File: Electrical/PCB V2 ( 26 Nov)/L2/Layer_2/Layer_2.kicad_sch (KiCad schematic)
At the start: 25 parts, among them SW1 SW_Push, U1 LM2596ADJ, U2 LM2596ADJ, U3 XT30UPB-M, U4 XT30UPB-M, U5 ESP32-S3-DEVKITM-1-N8, U6 XT30UPB-M, U7 XT30UPB-M, U8 XT30UPB-M, U9 XT30UPB-M

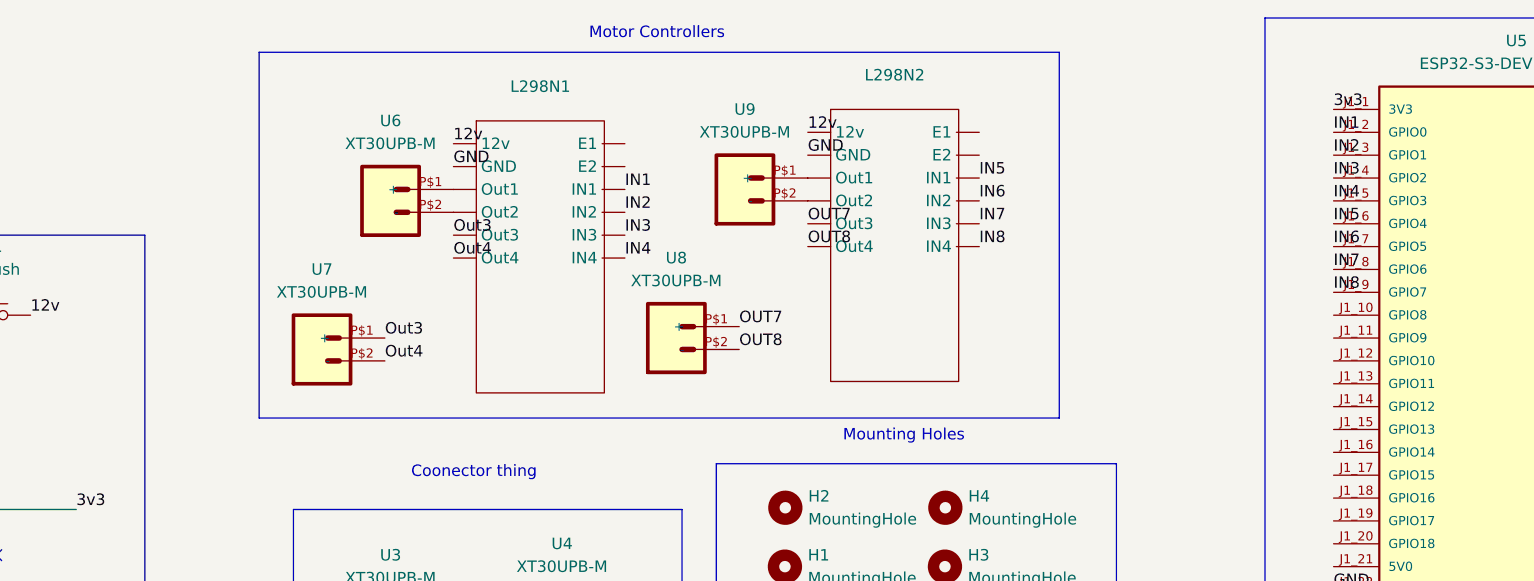
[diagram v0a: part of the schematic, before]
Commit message: concern
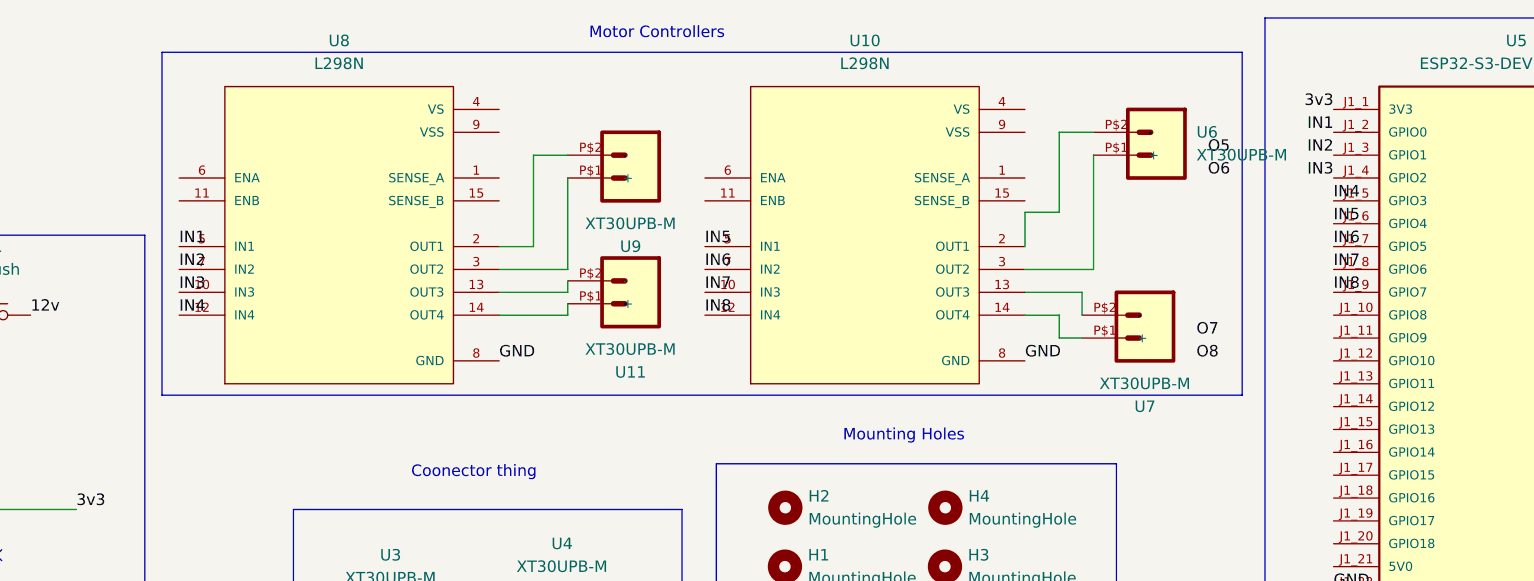
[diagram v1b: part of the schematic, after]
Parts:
- removed L298N1, L298N2: ~, l298n:TO127P2020X500X2100-15, symbol motor driver:L298N
- removed U8: XT30UPB-M, xt30:XT30UPB-M, symbol XT30UPB-M:XT30UPB-M
- added U10, U8: L298N, L298N:TO127P2020X500X2100-15, symbol l298n:L298N
- added U11: XT30UPB-M, xt30:XT30UPB-M, symbol XT30UPB-M:XT30UPB-M
- U3, U4: footprint XT30UPB-M:XT30UPB-M -> xt30:XT30UPB-M
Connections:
- net GND: now also U10.8 (GND), U8.8 (GND)
- net IN1: now also U8.5 (IN1)
- net IN2: now also U8.7 (IN2)
- net IN3: now also U8.10 (IN3)
- net IN4: now also U8.12 (IN4)
- net IN5: now also U10.5 (IN1)
- net IN6: now also U10.7 (IN2)
- net IN7: now also U10.10 (IN3)
- net IN8: now also U10.12 (IN4)
- net at U9.P$1 (+): now also U8.3 (OUT2)
- net at U9.P$2 (-): now also U8.2 (OUT1)
- net at U6.P$1 (+): now also U10.3 (OUT2)
- net at U6.P$2 (-): now also U10.2 (OUT1)
- net Out3: no longer names the net of U7.P$1 (+)
- net Out3: now also U10.14 (OUT4)
- net Out4: no longer names the net of U7.P$2 (-)
- net Out4: now also U10.13 (OUT3)
- new net: U11.P$1 (+), U8.14 (OUT4)
- new net: U11.P$2 (-), U8.13 (OUT3)
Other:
- moved on the sheet: U6, U7
